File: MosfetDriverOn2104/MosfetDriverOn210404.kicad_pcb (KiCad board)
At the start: 2 copper layers, 83.6 x 89.7 mm, 88 parts, among them J1 I2C HDR, J10 ENCODER HDR, J11 CROSS CONN, J12 motor, J2 AVR-ISP-6, J3 I2C HDR, J4 Screw_Terminal_01x02, J5 I2C HDR, J6 UART HDR, J7 5V HDR, J8 GND HDR, J9 servo hdr, Q1 IRF540N, Q2 IRF540N, Q3 IRF540N, Q4 IRF540N, SW1 SW_Push, SW2 SW_DIP_x04, SW3 SW_Push, SW4 SW_Push, U1 LM2576HVS-ADJ, U2 L7805, U3 IR2104, U4 LM358, U5 IR2104, U6 ATmega328P-AU-MCU_Microchip_A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

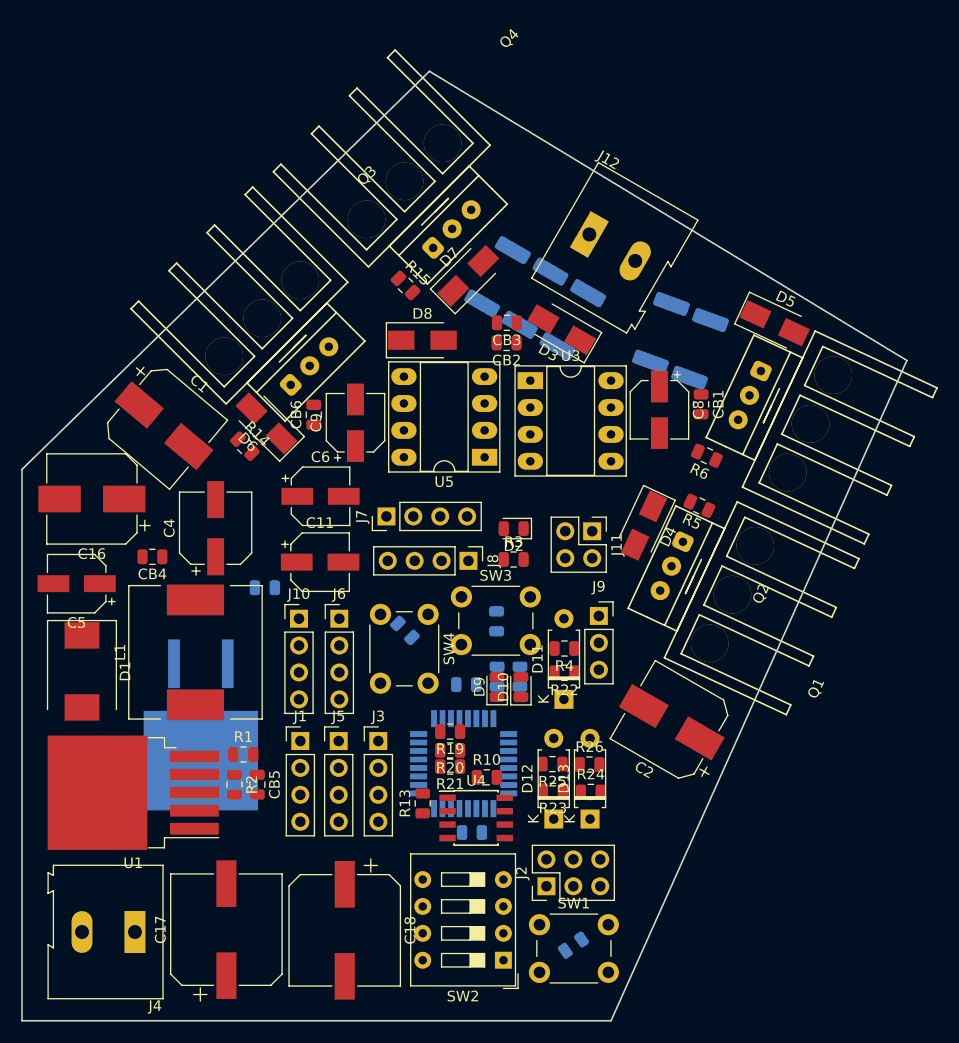
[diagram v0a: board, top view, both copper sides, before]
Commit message: Tested Route capability
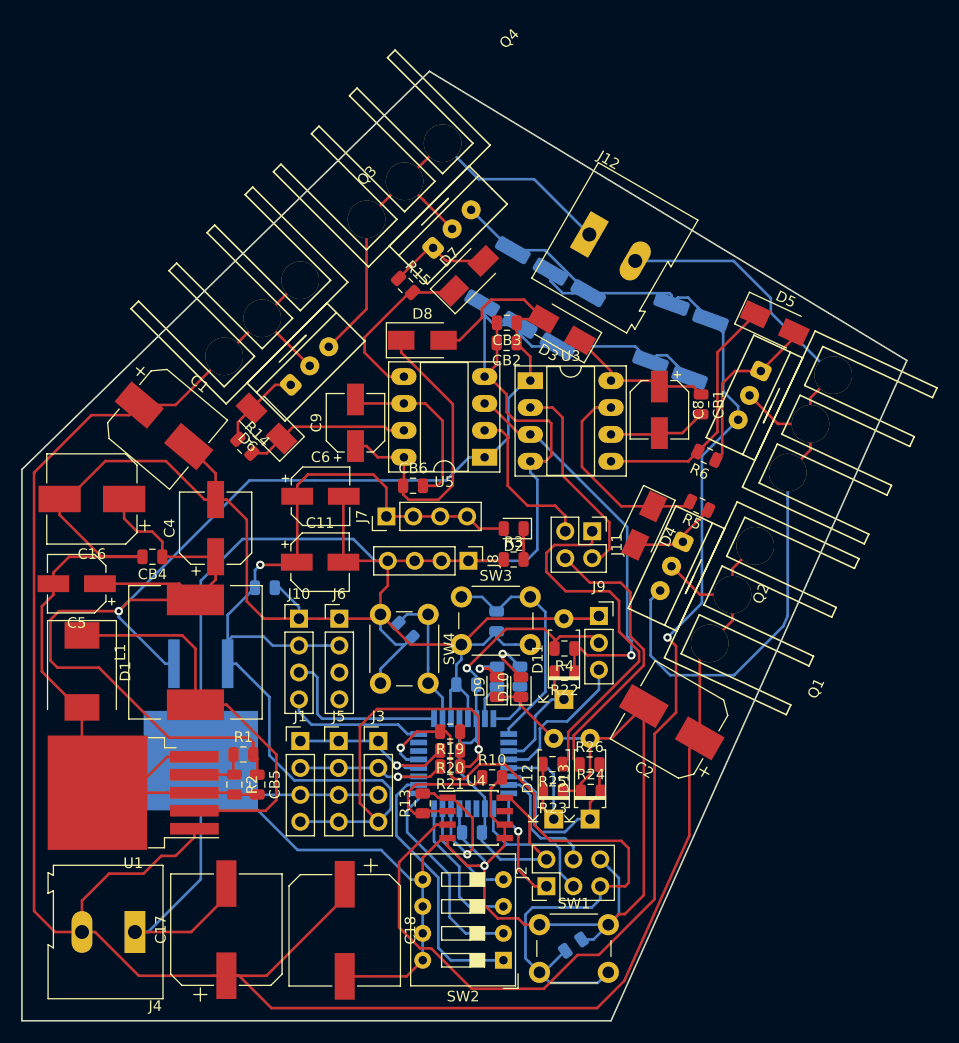
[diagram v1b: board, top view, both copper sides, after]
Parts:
- moved CB6 11.5 mm to (141.8, 100.7), turned to 0 degrees
- moved R10 0.51 mm to (149.3, 128.3)
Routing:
- net GND: track 0.00 -> 495.8 mm, vias 0 -> 1
- net VCC: track 0.00 -> 225.2 mm
- net +5V: track 0.00 -> 177.9 mm, vias 0 -> 3
- net +15V: track 0.00 -> 149.8 mm, vias 0 -> 1
- net /IS+: track 0.00 -> 134.7 mm, vias 0 -> 1
- net /M1: track 0.00 -> 78.1 mm
- net /RST: track 0.00 -> 65.8 mm, vias 0 -> 1
- net /M2: track 0.00 -> 47.6 mm
- net Net-(D1-Pad1): track 0.00 -> 38.6 mm
- net /~SD: track 0.00 -> 38.5 mm, vias 0 -> 1
- net /SGN1: track 0.00 -> 34.8 mm
- net Net-(C9-Pad1): track 0.00 -> 30.4 mm
- net /SGN2: track 0.00 -> 27.2 mm
- net Net-(SW2-Pad1): track 0.00 -> 25.2 mm
- net Net-(D5-Pad1): track 0.00 -> 23.8 mm
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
